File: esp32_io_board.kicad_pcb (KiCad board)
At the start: 2 copper layers, 60 parts, among them J1 USB_B_Micro, J11 Conn_01x02, J12 Conn_01x02, J13 Conn_01x02, J14 Conn_01x02, J2 Conn_02x04_Counter_Clockwise, J3 Conn_01x02, J4 Conn_01x02, J5 RASPBERRYPI-40-PIN-GPIO, J7 Conn_01x02, SW1 Reset, SW2 Bootloader, U1 CP2102N-A01-GQFN24, U4 ESP32-WROOM, U5 LM1117-3.3, U6 TCA9548APWR, U7 CAT24C256

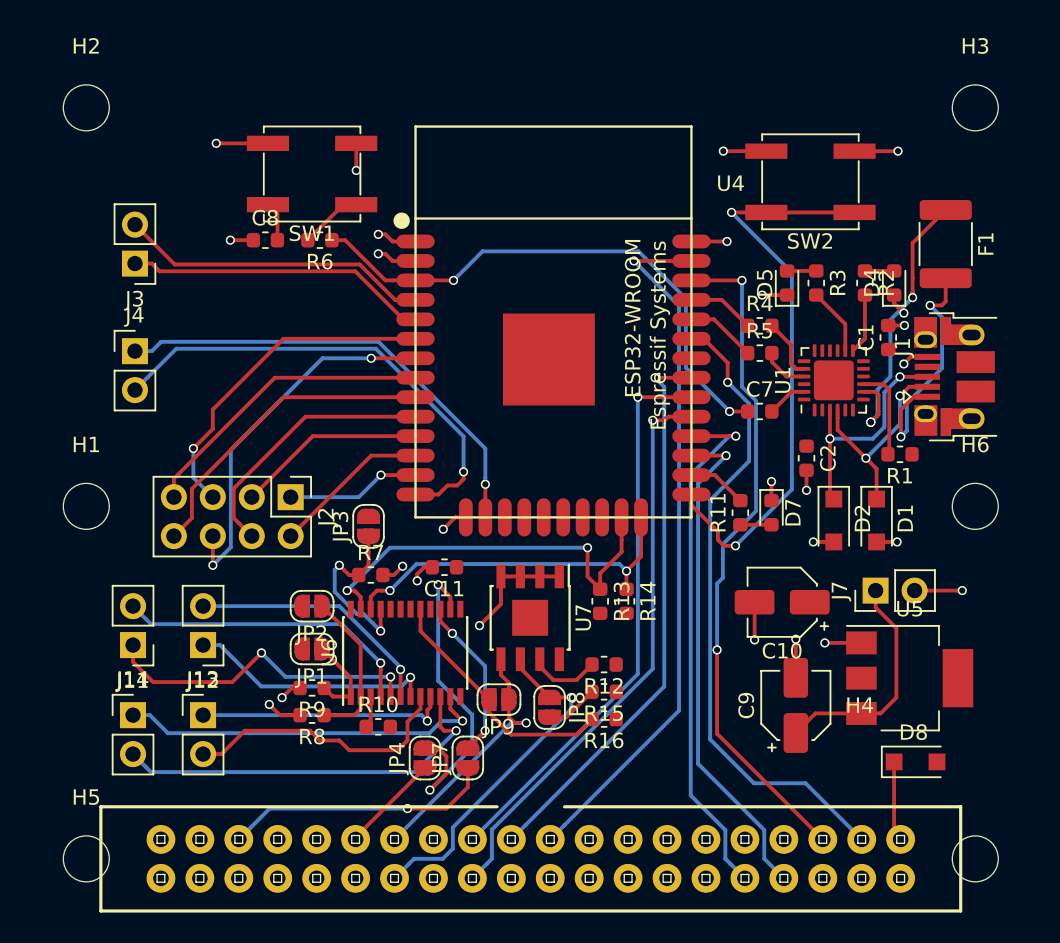
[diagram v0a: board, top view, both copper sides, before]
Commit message: layout design
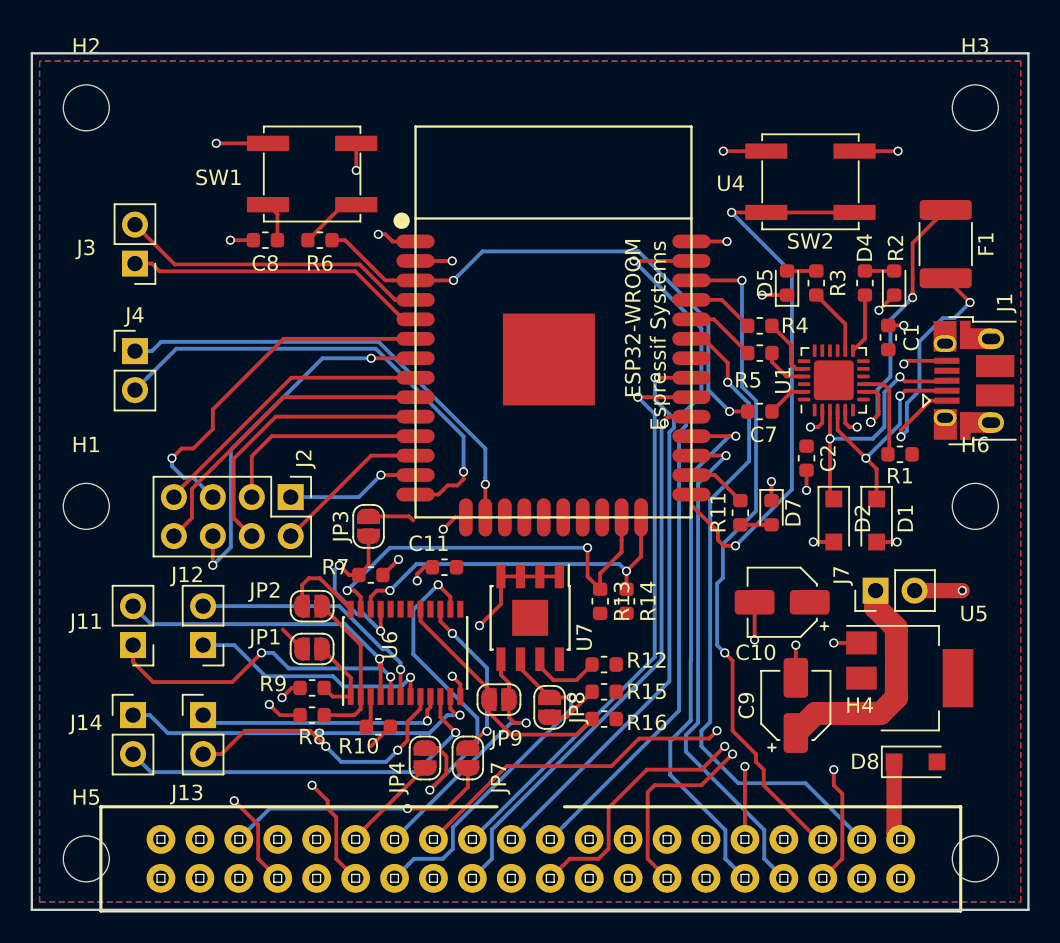
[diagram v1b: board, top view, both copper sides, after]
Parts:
- moved J1 1.30 mm to (217.9, 99.1)
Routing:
- net GND: track 55.5 -> 135.6 mm, vias 25 -> 34
- net +3V3: track 2.62 -> 16.3 mm, vias 1 -> 2
- net Net-(J2-Pad5): track 21.9 -> 23.9 mm
- net Net-(JP4-Pad2): track 21.7 -> 23.3 mm
- net Net-(J2-Pad3): track 12.3 -> 13.9 mm
- net Net-(D2-Pad1): track 15.3 -> 16.7 mm
- net /mosi: track 46.2 -> 47.4 mm
- net Net-(D1-Pad1): track 13.9 -> 15.0 mm
- net Net-(J2-Pad4): track 17.4 -> 18.5 mm
- net /tx: track 34.7 -> 35.8 mm
- net /sda0: track 41.8 -> 42.9 mm
- net +5V: track 16.5 -> 17.5 mm
- net /clk: track 36.8 -> 37.7 mm
- net /rx: track 32.9 -> 33.6 mm
- net Net-(J13-Pad2): track 18.0 -> 18.6 mm, vias 0 -> 2
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- added copper zone on F.Cu, net +3V3
- added copper zone on B.Cu, net GND
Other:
- board outline added: 65 x 55.9 mm
- net class power added: clearance 0.2, trace_width 1.5, via_dia 0.6, via_drill 0.4
